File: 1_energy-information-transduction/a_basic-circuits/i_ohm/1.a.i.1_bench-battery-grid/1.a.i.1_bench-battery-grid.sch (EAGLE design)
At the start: 2 parts

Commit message: Add lightbulb_with_pwm.txt.
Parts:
- added U$1, U$2, U$3: VOLTMETER, voltmeter:VOLTMETER
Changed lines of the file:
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@@
 <part name="GND1" library="supply1" deviceset="GND" device=""/>
 <part name="GND2" library="supply1" deviceset="GND" device=""/>
+<part name="U$1" library="voltmeter" deviceset="VOLTMETER" device=""/>
+<part name="U$2" library="voltmeter" deviceset="VOLTMETER" device=""/>
+<part name="U$3" library="voltmeter" deviceset="VOLTMETER" device=""/>
 </parts>
 <sheets>

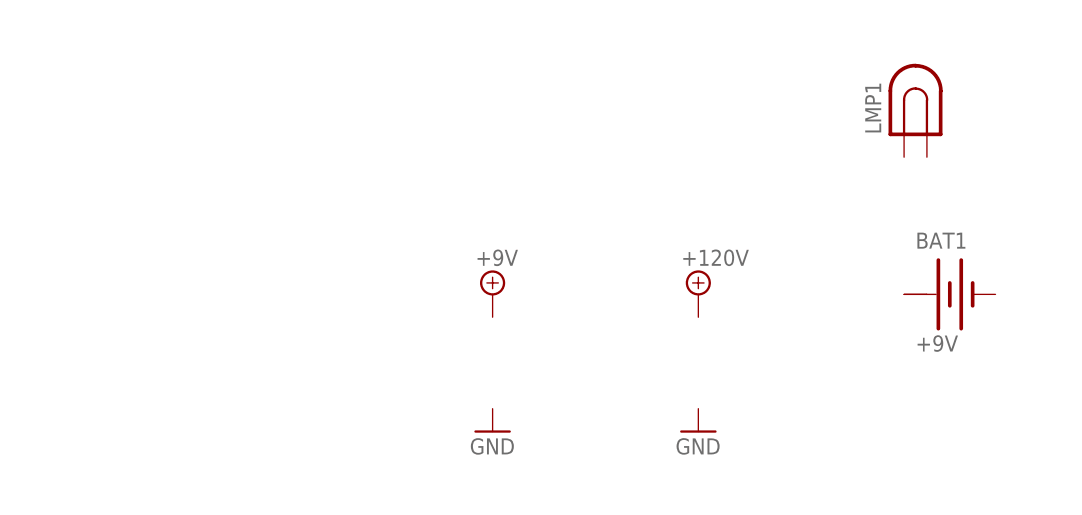
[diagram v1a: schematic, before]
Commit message: Update 1.a.i.1.
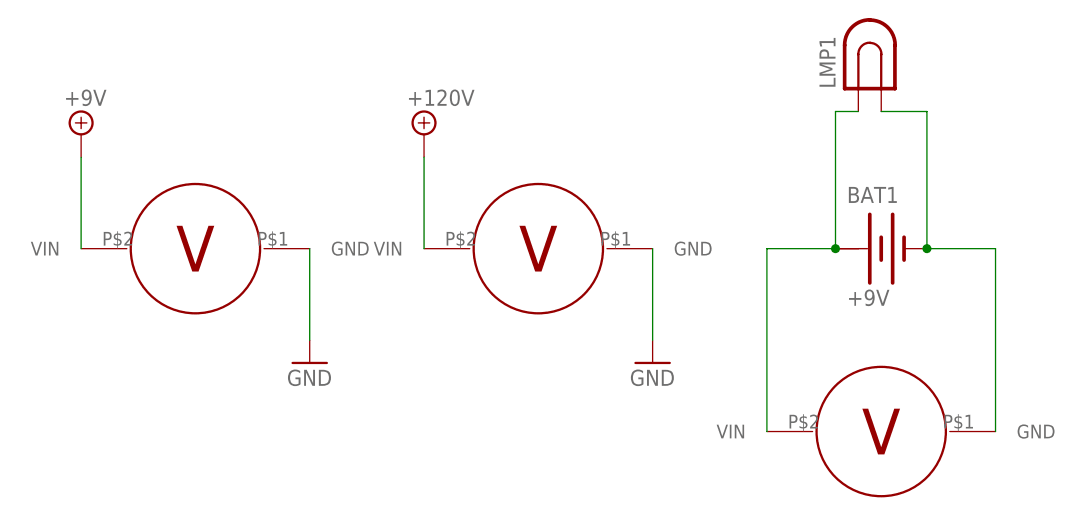
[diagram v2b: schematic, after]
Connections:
- new net N$1: BAT1.+, LMP1.1
- new net N$2: BAT1.-, LMP1.2
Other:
- moved on the sheet: BAT1, LMP1
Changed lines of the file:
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@@
 <layer number="93" name="Pins" color="2" fill="1" visible="no" active="yes"/>
 <layer number="94" name="Symbols" color="4" fill="1" visible="yes" active="yes"/>
-<layer number="95" name="Names" color="7" fill="1" visible="yes" active="yes"/>
+<layer number="95" name="Names" color="7" fill="1" visible="no" active="yes"/>
 <layer number="96" name="Values" color="7" fill="1" visible="yes" active="yes"/>
 <layer number="97" name="Info" color="7" fill="1" visible="yes" active="yes"/>
@@
 </plain>
 <instances>
-<instance part="SUPPLY1" gate="G$1" x="22.86" y="45.72"/>
-<instance part="LMP1" gate="G$1" x="68.58" y="66.04"/>
-<instance part="SUPPLY2" gate="G$1" x="45.72" y="45.72"/>
-<instance part="BAT1" gate="G$1" x="73.66" y="45.72"/>
-<instance part="GND1" gate="1" x="22.86" y="30.48"/>
-<instance part="GND2" gate="1" x="45.72" y="30.48"/>
+<instance part="SUPPLY1" gate="G$1" x="-22.86" y="63.5"/>
+<instance part="LMP1" gate="G$1" x="63.5" y="71.12"/>
+<instance part="SUPPLY2" gate="G$1" x="15.24" y="63.5"/>
+<instance part="BAT1" gate="G$1" x="66.04" y="50.8"/>
+<instance part="GND1" gate="1" x="2.54" y="38.1"/>
+<instance part="GND2" gate="1" x="40.64" y="38.1"/>
+<instance part="U$1" gate="G$1" x="66.04" y="30.48"/>
+<instance part="U$2" gate="G$1" x="27.94" y="50.8"/>
+<instance part="U$3" gate="G$1" x="-10.16" y="50.8"/>
 </instances>
 <busses>
 </busses>
 <nets>
+<net name="+9V" class="0">
+<segment>
+<pinref part="SUPPLY1" gate="G$1" pin="+9V"/>
+<wire x1="-22.86" y1="60.96" x2="-22.86" y2="50.8" width="0.1524" layer="91"/>
+</segment>
+<segment>
+<pinref part="SUPPLY2" gate="G$1" pin="+9V"/>
+<wire x1="15.24" y1="60.96" x2="15.24" y2="50.8" width="0.1524" layer="91"/>
+</segment>
+</net>
+<net name="GND" class="0">
+<segment>
+<pinref part="GND1" gate="1" pin="GND"/>
+<wire x1="2.54" y1="50.8" x2="2.54" y2="40.64" width="0.1524" layer="91"/>
+</segment>
+<segment>
+<pinref part="GND2" gate="1" pin="GND"/>
+<wire x1="40.64" y1="50.8" x2="40.64" y2="40.64" width="0.1524" layer="91"/>
+</segment>
+</net>
+<net name="N$1" class="0">
+<segment>
+<pinref part="BAT1" gate="G$1" pin="+"/>
+<wire x1="60.96" y1="50.8" x2="60.96" y2="66.04" width="0.1524" layer="91"/>
+<pinref part="LMP1" gate="G$1" pin="1"/>
+<wire x1="60.96" y1="66.04" x2="63.5" y2="66.04" width="0.1524" layer="91"/>
+<wire x1="53.34" y1="30.48" x2="53.34" y2="50.8" width="0.1524" layer="91"/>
+<wire x1="53.34" y1="50.8" x2="60.96" y2="50.8" width="0.1524" layer="91"/>
+<junction x="60.96" y="50.8"/>
+</segment>
+</net>
+<net name="N$2" class="0">
+<segment>
+<pinref part="BAT1" gate="G$1" pin="-"/>
+<wire x1="71.12" y1="50.8" x2="71.12" y2="66.04" width="0.1524" layer="91"/>
+<pinref part="LMP1" gate="G$1" pin="2"/>
+<wire x1="71.12" y1="66.04" x2="66.04" y2="66.04" width="0.1524" layer="91"/>
+<wire x1="78.74" y1="30.48" x2="78.74" y2="50.8" width="0.1524" layer="91"/>
+<wire x1="78.74" y1="50.8" x2="71.12" y2="50.8" width="0.1524" layer="91"/>
+<junction x="71.12" y="50.8"/>
+</segment>
+</net>
 </nets>
 </sheet>
